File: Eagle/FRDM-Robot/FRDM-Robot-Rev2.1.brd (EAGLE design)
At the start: 92.8 x 65 mm, 49 parts

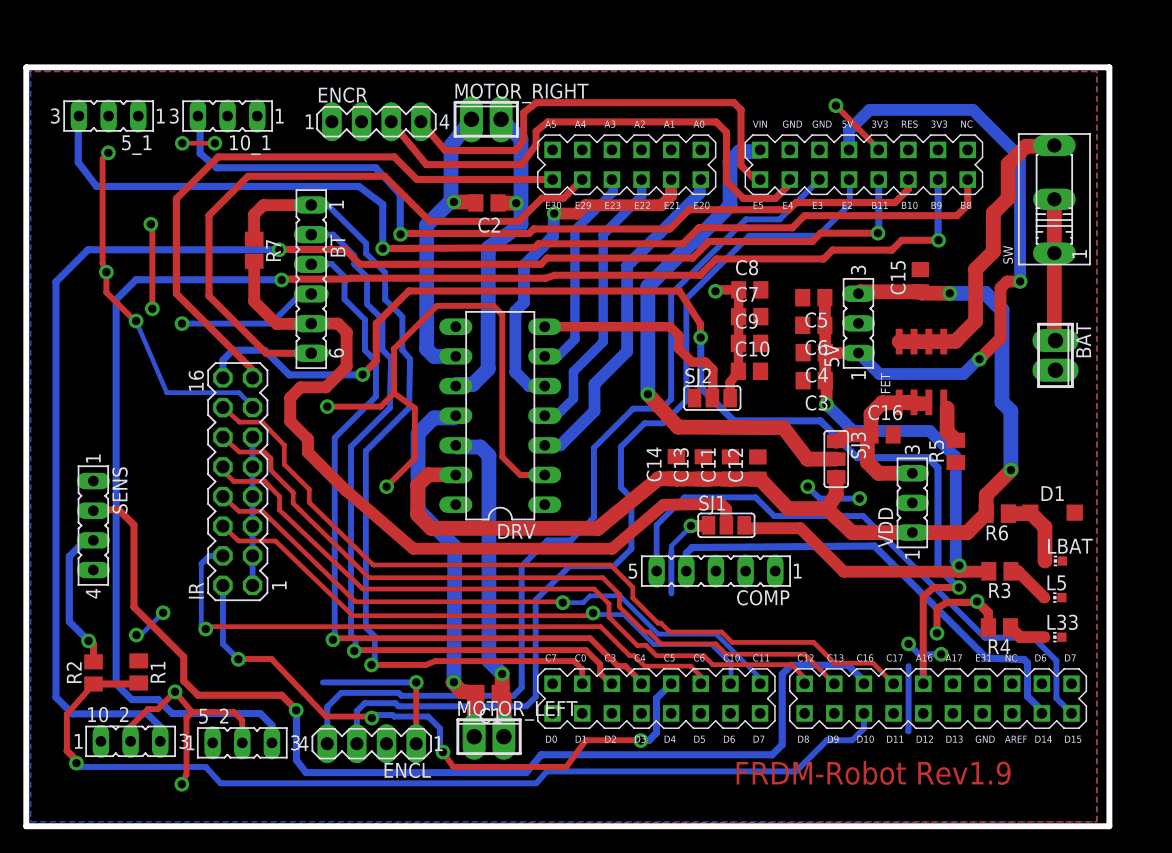
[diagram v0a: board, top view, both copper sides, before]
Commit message: new rev 2.1 of FRDM-Robot
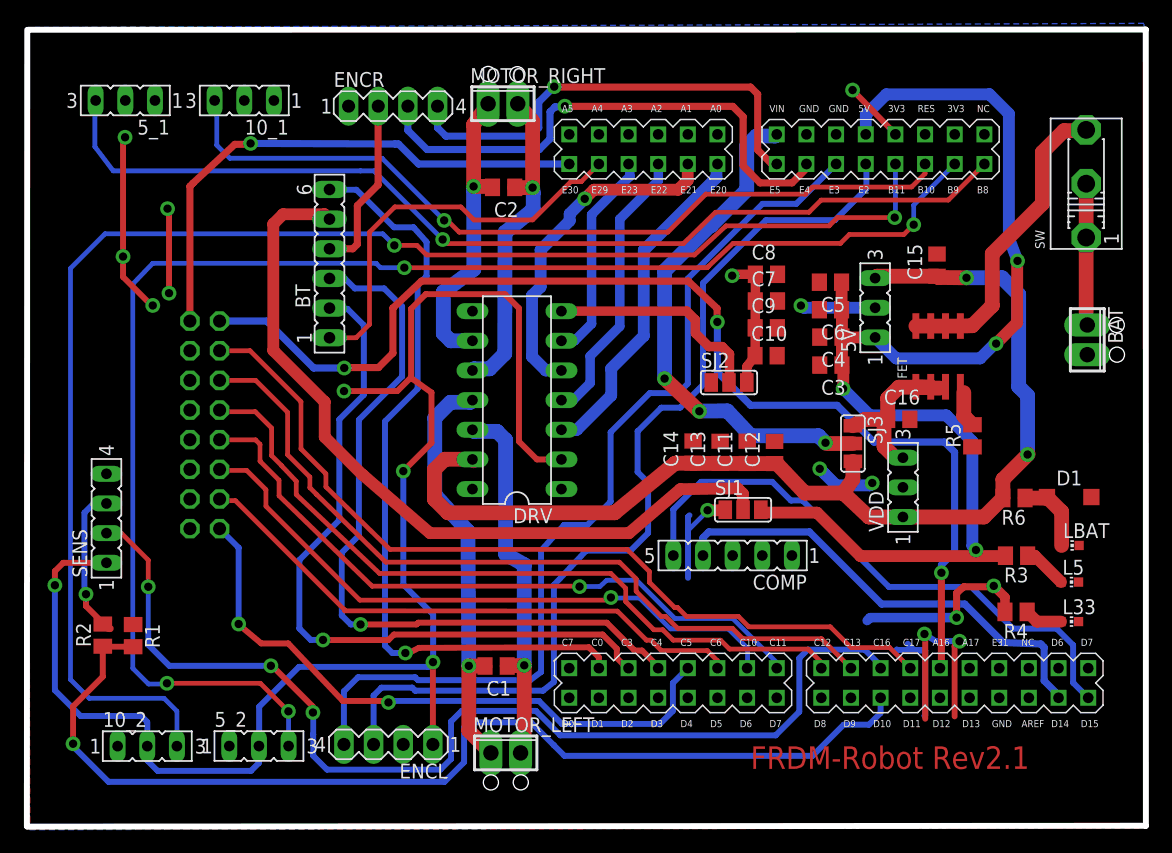
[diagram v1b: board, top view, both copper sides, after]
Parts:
- removed R7: 10k, resistor:M0805
- R3: value 220 -> 470
- R4: value 150 -> 330
- R6: value 470 -> 2k2
- moved IR 5.63 mm to (15.5, 34.6), flipped to the bottom
- moved SENS 3.35 mm to (7.12, 27.9), turned to 90 degrees
- moved R2 3.34 mm to (6.80, 16.6)
- moved R1 3.15 mm to (9.40, 16.6)
- moved BAT 3.03 mm to (91.1, 41.9)
- moved SW 3.03 mm to (91.0, 55.3)
- moved C1 2.45 mm to (40.5, 14.0)
- moved BT 2.05 mm to (26.2, 48.4), turned to 90 degrees
- moved MOTOR_LEFT 1.99 mm to (41.3, 6.54)
- moved 5V 1.95 mm to (73.0, 44.7)
- moved C15 1.95 mm to (78.3, 48.3)
- moved C16 1.95 mm to (75.0, 35.1)
- moved FET 1.95 mm to (78.3, 40.5)
- moved L33 1.95 mm to (89.6, 17.8)
- moved L5 1.95 mm to (89.6, 21.2)
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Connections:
- net KEY: now also BT.6; no longer BT.1, R7.1
- net STATE: now also BT.1; no longer BT.6
- net VCC: no longer R7.2
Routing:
- net +3V3: track 162.8 -> 207.6 mm, vias 17 -> 14
- net STATE: track 54.1 -> 34.8 mm
- net GND: track 36.0 -> 43.6 mm, vias 7 -> 5
- net ECHO: track 83.4 -> 90.4 mm
- net IR_LED_ON: track 52.7 -> 46.2 mm, vias 0 -> 1
- net KEY: track 72.7 -> 66.2 mm
- net BOUT2: track 28.1 -> 32.9 mm
- net IR_REF_5: track 53.3 -> 58.1 mm
- net IR_REF_3: track 62.8 -> 67.5 mm
- net IR_REF_2: track 69.3 -> 73.9 mm
- net IR_REF_6: track 50.0 -> 54.4 mm
- net IR_REF_4: track 59.3 -> 63.6 mm
- net IR_REF_7: track 53.0 -> 49.0 mm, vias 1 -> 0
- net BOUT1: track 32.9 -> 35.9 mm
- net BTRX: track 64.9 -> 62.3 mm
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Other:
- board size 92.8 x 65 mm -> 95.8 x 68.3 mm
- board text added: "FRDM-Robot Rev2.1"
- board text removed: "FRDM-Robot Rev1.9"
